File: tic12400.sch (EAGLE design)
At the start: 21 parts, among them X1 22-23-2031

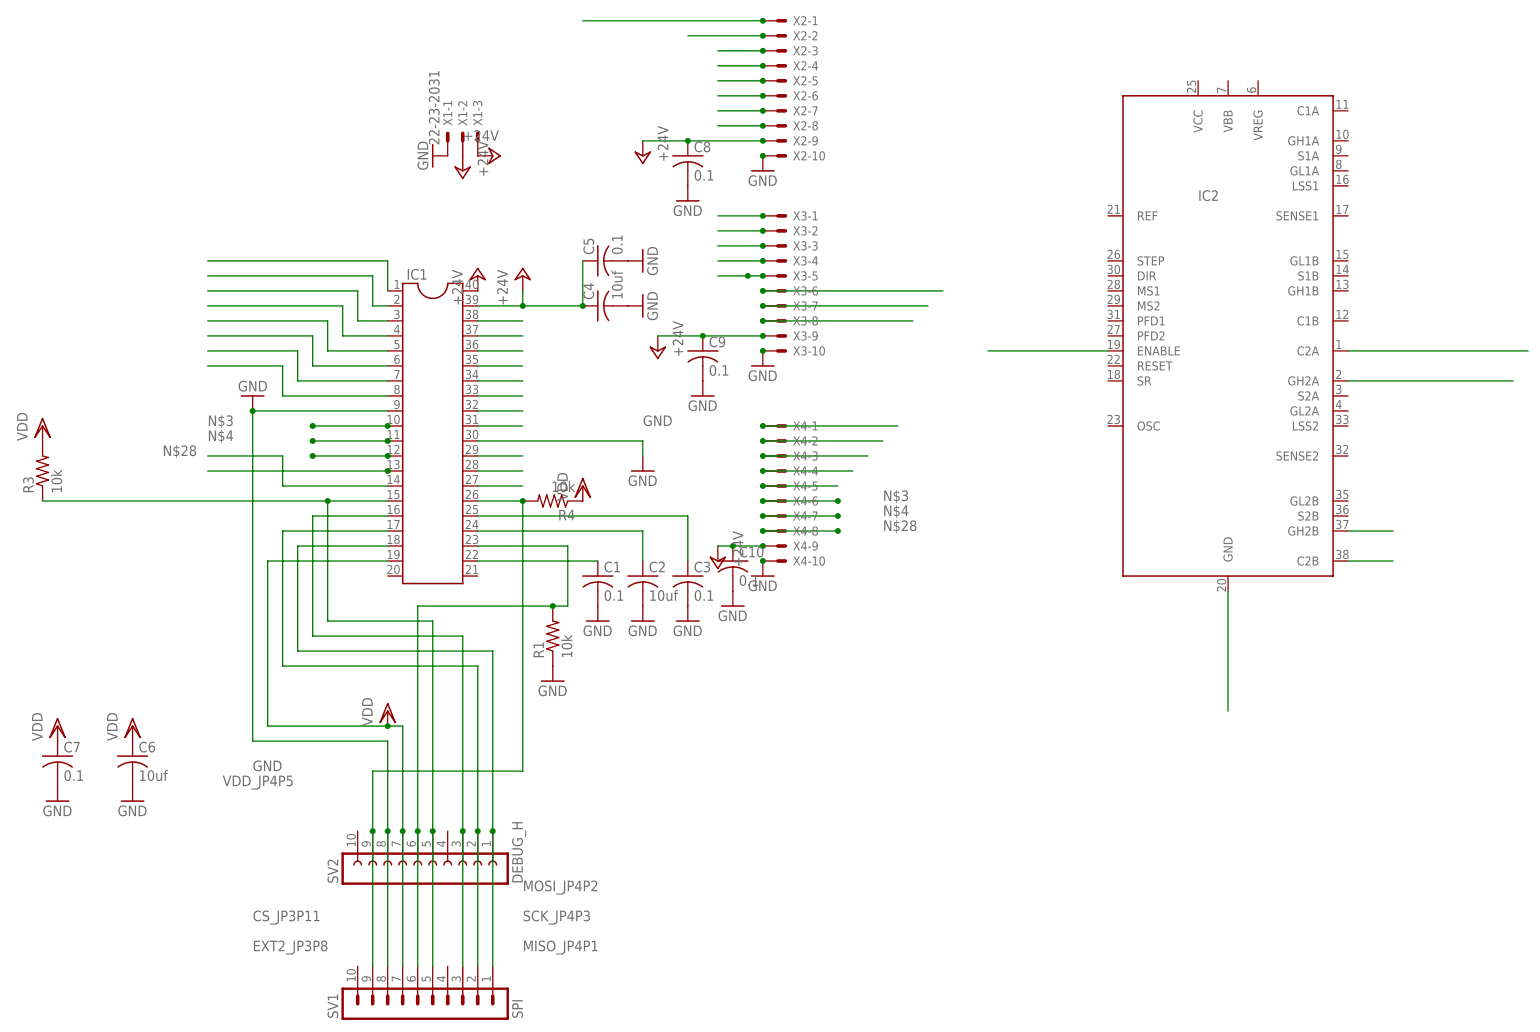
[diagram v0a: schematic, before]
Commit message: up
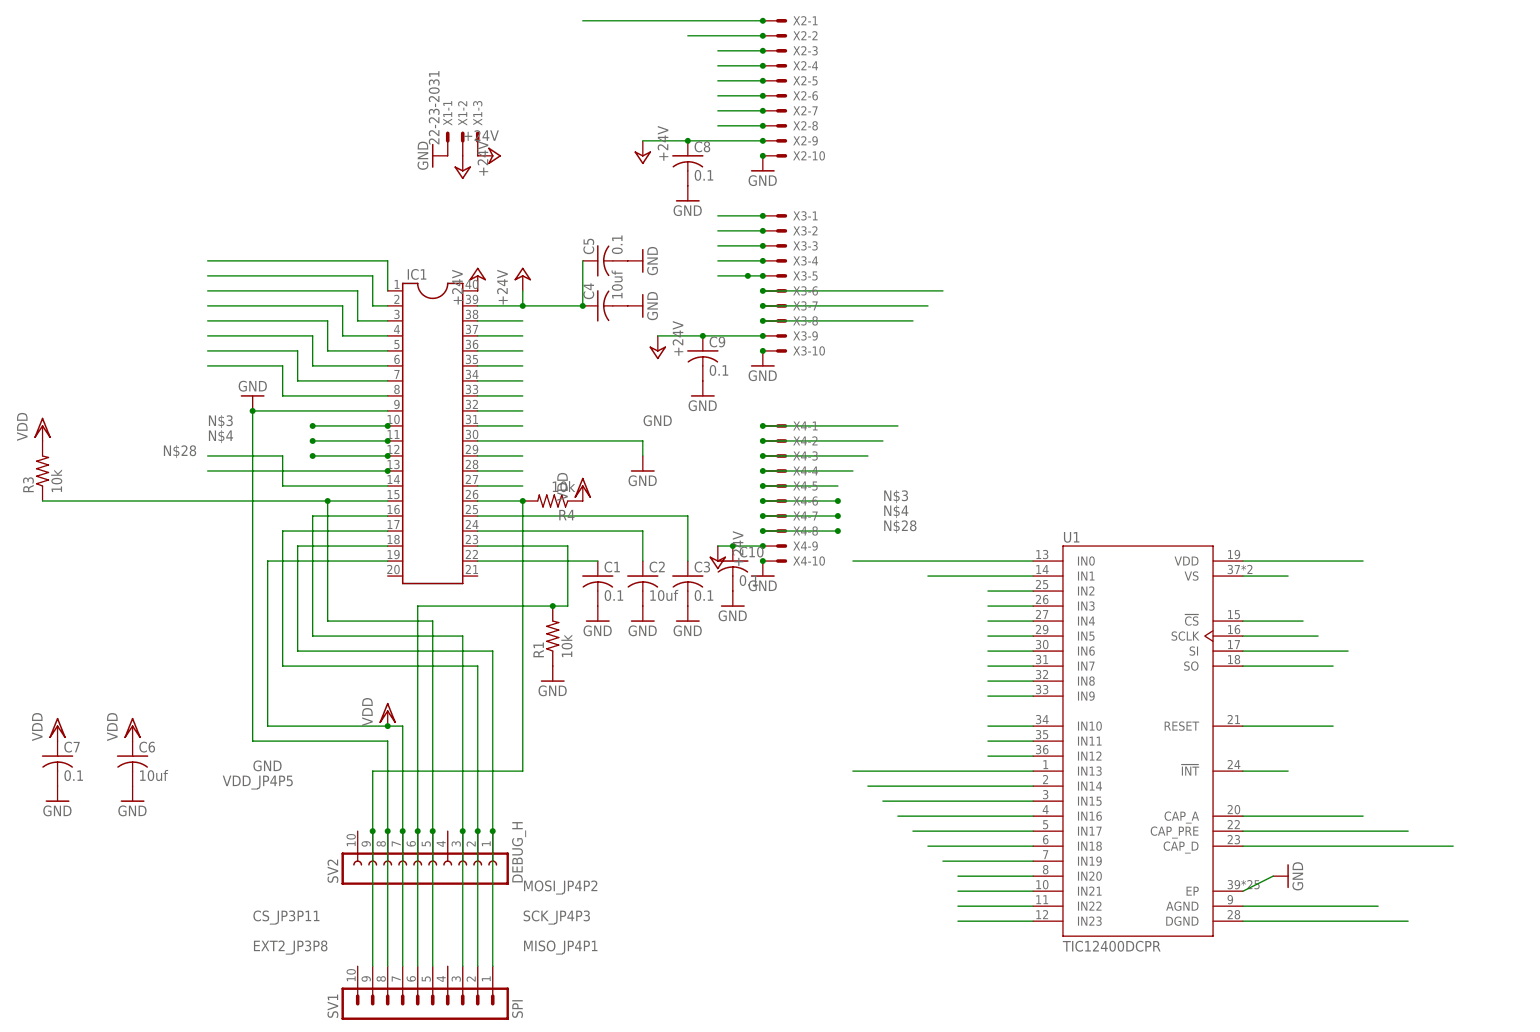
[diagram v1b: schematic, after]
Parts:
- removed IC2: (no value), allegro2:A3986
- added U1: TIC12400DCPR, TIC12400DCPR:TIC12400DCPR
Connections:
- net +24V: no longer IC2.C2B, IC2.GH2B
- net CS_JP3P11: now also U1.!CS
- net EXT2_JP3P8: now also U1.!INT
- net GND: now also U1.AGND, U1.DGND, U1.EP
- net MISO_JP4P1: now also U1.SO
- net MOSI_JP4P2: now also U1.SCLK
- net N$1: now also U1.IN0
- net N$10: now also U1.CAP_D
- net N$11: now also U1.IN18
- net N$12: now also U1.IN17
- net N$13: now also U1.IN16
- net N$14: now also U1.IN15
- net N$15: now also U1.IN14; no longer IC2.GH2A
- net N$16: now also U1.IN13; no longer IC2.C2A
- net N$17: now also U1.IN2
- net N$18: now also U1.IN3
- net N$19: now also U1.IN4
- net N$2: now also U1.IN1
- net N$20: now also U1.IN5
- net N$21: now also U1.IN6
- net N$22: now also U1.IN7
- net N$23: now also U1.IN8
- net N$24: now also U1.IN9
- net N$25: now also U1.IN10
- net N$26: now also U1.IN11
- net N$27: now also U1.IN12, U1.VS
- net N$28: now also U1.IN23
- net N$3: now also U1.IN21
- net N$4: now also U1.IN22
- net N$5: now also U1.IN20
- net N$6: now also U1.RESET
- net N$7: now also U1.IN19
- net N$8: now also U1.CAP_A; no longer IC2.GND
- net N$9: now also U1.CAP_PRE
- net SCK_JP4P3: now also U1.SI
- net VDD_JP4P5: now also U1.VDD; no longer IC2.ENABLE
